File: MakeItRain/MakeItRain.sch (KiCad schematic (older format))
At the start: 19 parts, among them IC1 LM2597MX-5.0_NOPB, IC2 TL071CP, J10 Conn_01x15, J11 Conn_01x15, P1 Screw_Terminal_01x02, Q1 IRF9Z34NPBF, U1 178.6165.0001

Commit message: WIP to test some hardware designs.
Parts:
- removed IC2: TL071CP, SamacSys_Parts:DIP794W53P254L959H508Q8N, symbol SamacSys_Parts:TL071CP
- removed J10, J11: Conn_01x15, Connector_PinSocket_2.54mm:PinSocket_1x15_P2.54mm_Vertical, symbol Connector_Generic:Conn_01x15
- added IC2: OPA2340PA, DIP794W53P254L959H508Q8N, symbol SamacSys_Parts:OPA2340PA
- added J1, J2: Conn_01x19, Connector_PinSocket_2.54mm:PinSocket_1x19_P2.54mm_Vertical, symbol Connector_Generic:Conn_01x19
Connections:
- net labels added: +5V, 3.3V, 5V, CLK, P0, P15, P16, P17, P18, P19, P2, P21, P22, P23, P4, P5, RX, SD1, SD2, SD3, SDD, SVN, SVP, TX
- net labels removed: 3v3, D15, D18, D19, D2, D21, D22, D23, D4, D5, RX0, RX2, TX0, TX2, VN, VP, Vin
- wire segments 61 -> 122
- no-connect marks 2 -> 17
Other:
- moved on the sheet: IC1, R26, R27, R28

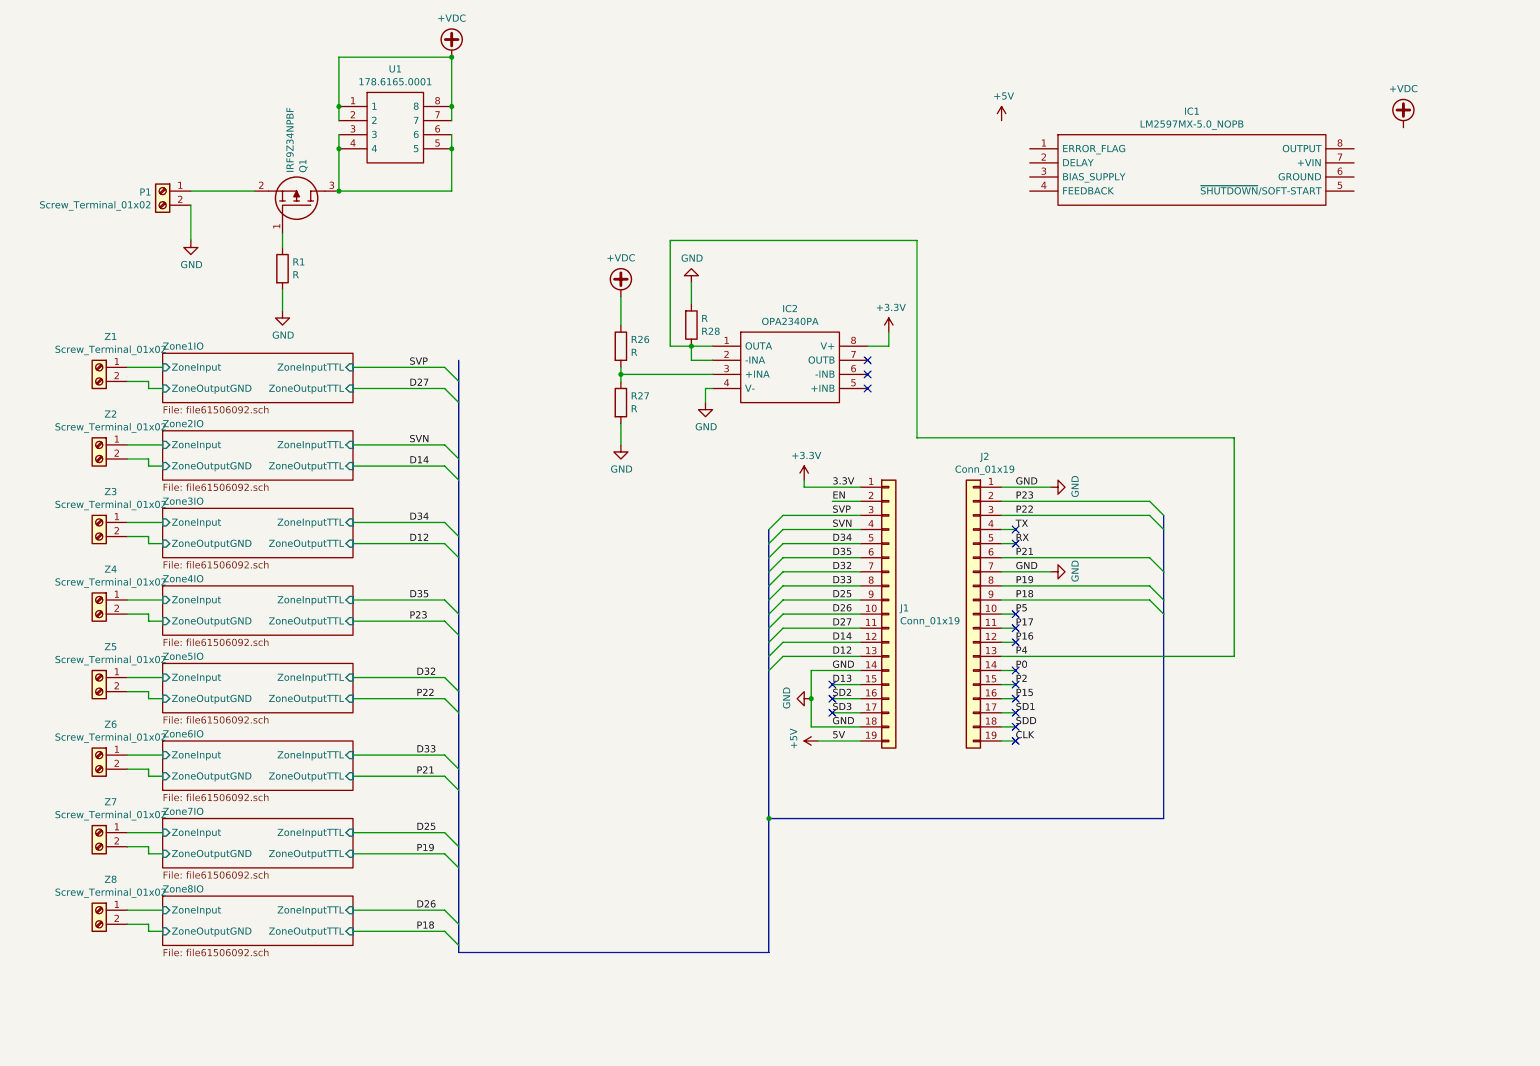
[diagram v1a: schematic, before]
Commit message: wip for layout
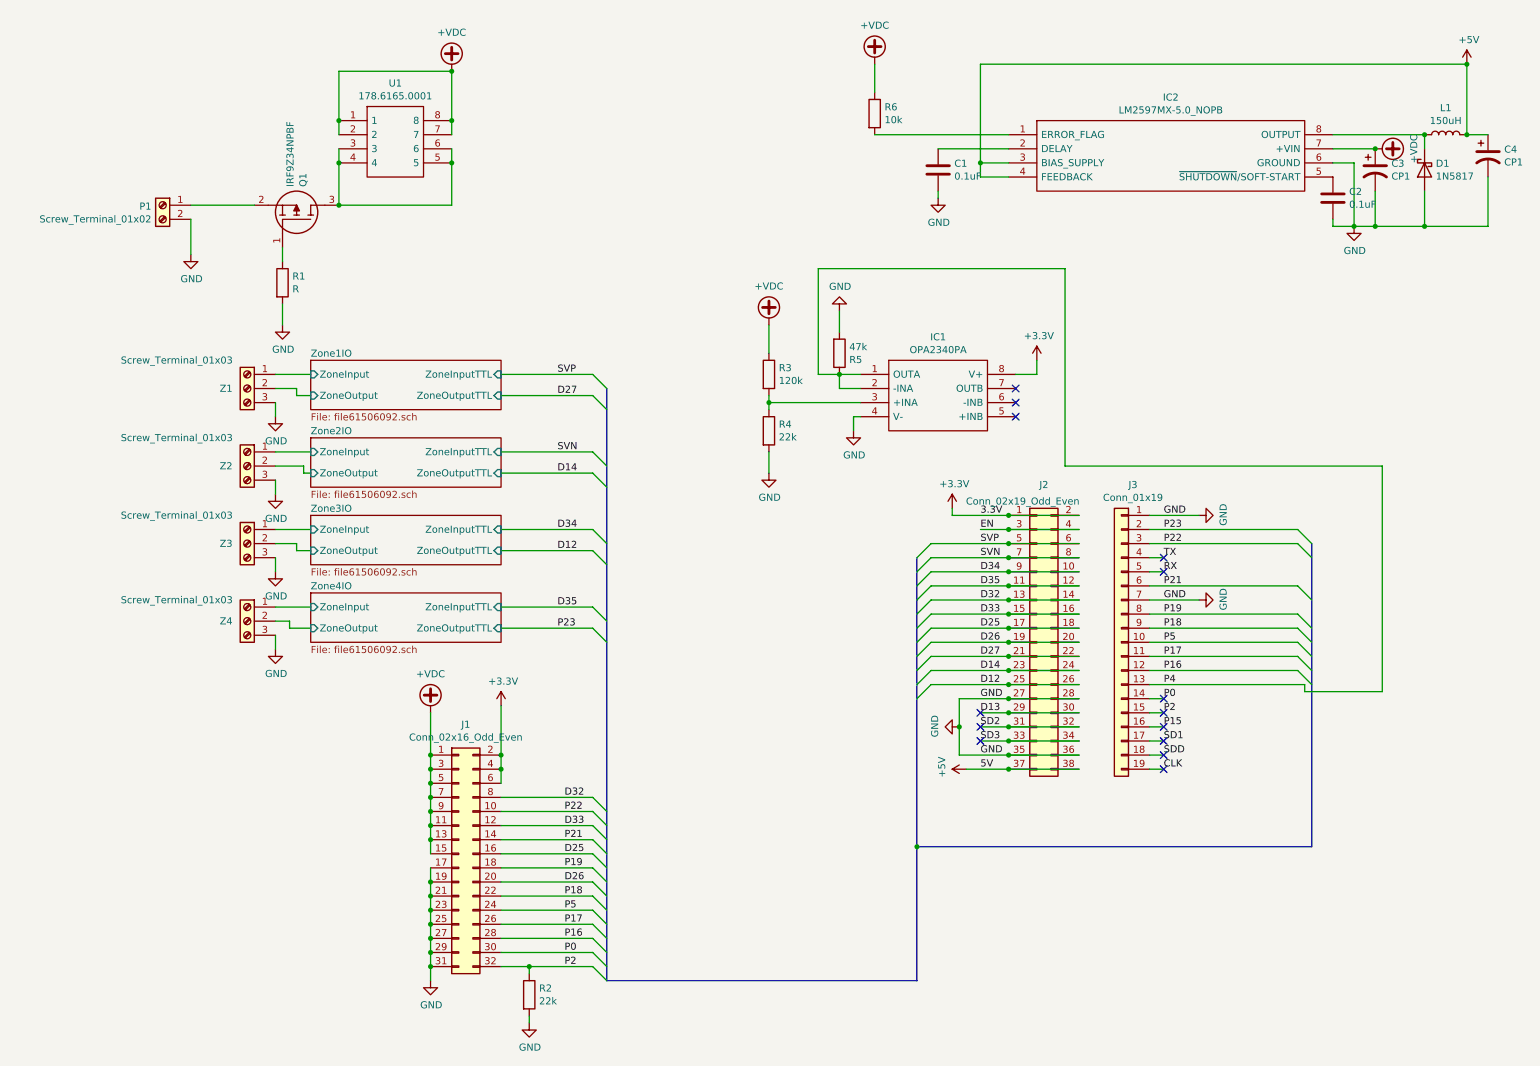
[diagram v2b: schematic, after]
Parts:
- removed J1: Conn_01x19, Connector_PinSocket_2.54mm:PinSocket_1x19_P2.54mm_Vertical, symbol Connector_Generic:Conn_01x19
- removed Z1, Z2, Z3, Z4, Z5, Z6, Z7, Z8: Screw_Terminal_01x02, TerminalBlock_Phoenix:TerminalBlock_Phoenix_MKDS-1,5-2-5.08_1x02_P5.08mm_Horizontal, symbol Connector:Screw_Terminal_01x02
- added C1, C2: 0.1uF, Capacitor_THT:C_Disc_D4.7mm_W2.5mm_P5.00mm, symbol Device:C
- added C3, C4: CP1, Capacitor_THT:CP_Radial_D8.0mm_P3.50mm, symbol Device:CP1
- added D1: 1N5817, Diode_THT:D_DO-41_SOD81_P10.16mm_Horizontal, symbol Diode:1N5817
- added J1: Conn_02x16_Odd_Even, Connector_PinHeader_2.54mm:PinHeader_2x16_P2.54mm_Vertical, symbol Connector_Generic:Conn_02x16_Odd_Even
- added J2: Conn_02x19_Odd_Even, Connector_PinSocket_2.54mm:PinSocket_2x19_P2.54mm_Vertical, symbol Connector_Generic:Conn_02x19_Odd_Even
- added L1: 150uH, Inductor_THT:L_Axial_L6.6mm_D2.7mm_P10.16mm_Horizontal_Vishay_IM-2, symbol Device:L
- added R2: 22k, Resistor_THT:R_Axial_DIN0207_L6.3mm_D2.5mm_P5.08mm_Vertical, symbol Device:R
- added R6: 10k, Resistor_THT:R_Axial_DIN0207_L6.3mm_D2.5mm_P5.08mm_Vertical, symbol Device:R
- added Z1, Z2, Z3, Z4: Screw_Terminal_01x03, TerminalBlock_Phoenix:TerminalBlock_Phoenix_MKDS-1,5-3-5.08_1x03_P5.08mm_Horizontal, symbol Connector:Screw_Terminal_01x03
- IC1: renamed from IC2; footprint DIP794W53P254L959H508Q8N -> SamacSys_Parts:DIP794W53P254L959H508Q8N
- R3: renamed from R26; value R -> 120k
- R4: renamed from R27; value R -> 22k
- R5: renamed from R28; value R -> 47k
- renumbered IC1 to IC2, J2 to J3
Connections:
- net +3V3: now also J1.2 (Pin_2), J1.4 (Pin_4), J1.6 (Pin_6), J2.1 (Pin_1), J2.2 (Pin_2)
- net +5V: now also IC2.3 (BIAS_SUPPLY), IC2.4 (FEEDBACK), C4.1, J2.37 (Pin_37), J2.38 (Pin_38), L1.2
- net +VDC: now also IC2.7 (+VIN), C3.1, J1.1 (Pin_1), J1.11 (Pin_11), J1.13 (Pin_13), J1.15 (Pin_15), J1.3 (Pin_3), J1.5 (Pin_5), J1.7 (Pin_7), J1.9 (Pin_9), R6.1
- net D12: now also J2.25 (Pin_25), J2.26 (Pin_26)
- net D13: now also J2.29 (Pin_29), J2.30 (Pin_30)
- net D14: now also J2.23 (Pin_23), J2.24 (Pin_24)
- net D25: now also J1.16 (Pin_16), J2.17 (Pin_17), J2.18 (Pin_18)
- net D26: now also J1.20 (Pin_20), J2.19 (Pin_19), J2.20 (Pin_20)
- net D27: now also J2.21 (Pin_21), J2.22 (Pin_22)
- net D32: now also J1.8 (Pin_8), J2.13 (Pin_13), J2.14 (Pin_14)
- net D33: now also J1.12 (Pin_12), J2.15 (Pin_15), J2.16 (Pin_16)
- net D34: now also J2.10 (Pin_10), J2.9 (Pin_9)
- net D35: now also J2.11 (Pin_11), J2.12 (Pin_12)
- net EN: now also J2.3 (Pin_3), J2.4 (Pin_4)
- net GND: now also IC2.6 (GROUND), C1.2, C2.2, C3.2, C4.2, D1.2 (A), J1.17 (Pin_17), J1.19 (Pin_19), J1.21 (Pin_21), J1.23 (Pin_23), J1.25 (Pin_25), J1.27 (Pin_27), J1.29 (Pin_29), J1.31 (Pin_31), J2.27 (Pin_27), J2.28 (Pin_28), J2.35 (Pin_35), J2.36 (Pin_36), R2.2, Z1.3 (Pin_3), Z2.3 (Pin_3), Z3.3 (Pin_3), Z4.3 (Pin_3)
- net P0: now also J1.30 (Pin_30)
- net P16: now also J1.28 (Pin_28)
- net P17: now also J1.26 (Pin_26)
- net P18: now also J1.22 (Pin_22)
- net P19: now also J1.18 (Pin_18)
- net P2: now also J1.32 (Pin_32), R2.1
- net P21: now also J1.14 (Pin_14)
- net P22: now also J1.10 (Pin_10)
- net P5: now also J1.24 (Pin_24)
- net SD2: now also J2.31 (Pin_31), J2.32 (Pin_32)
- net SD3: now also J2.33 (Pin_33), J2.34 (Pin_34)
- net SVN: now also J2.7 (Pin_7), J2.8 (Pin_8)
- net SVP: now also J2.5 (Pin_5), J2.6 (Pin_6)
- net Zone1IO/ZoneInput: now also Z1.1 (Pin_1)
- net Zone2IO/ZoneInput: now also Z2.1 (Pin_1)
- net Zone3IO/ZoneInput: now also Z3.1 (Pin_1)
- net Zone4IO/ZoneInput: now also Z4.1 (Pin_1)
- net at IC2.1 (ERROR_FLAG): now also R6.2
- net at IC2.2 (DELAY): now also C1.1
- net at IC2.5 (~SHUTDOWN~/SOFT-START): now also C2.1
- net at IC2.8 (OUTPUT): now also D1.1 (K), L1.1
- new net Zone1IO/ZoneOutput: Z1.2 (Pin_2)
- new net Zone2IO/ZoneOutput: Z2.2 (Pin_2)
- new net Zone3IO/ZoneOutput: Z3.2 (Pin_2)
- new net Zone4IO/ZoneOutput: Z4.2 (Pin_2)
- no-connect marks 17 -> 14
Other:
- moved on the sheet: IC1, IC2, J3, P1, Q1, R1, R3, R4, R5, U1
